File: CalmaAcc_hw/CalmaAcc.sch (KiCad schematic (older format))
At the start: 27 parts, among them Q1 MMBT2222

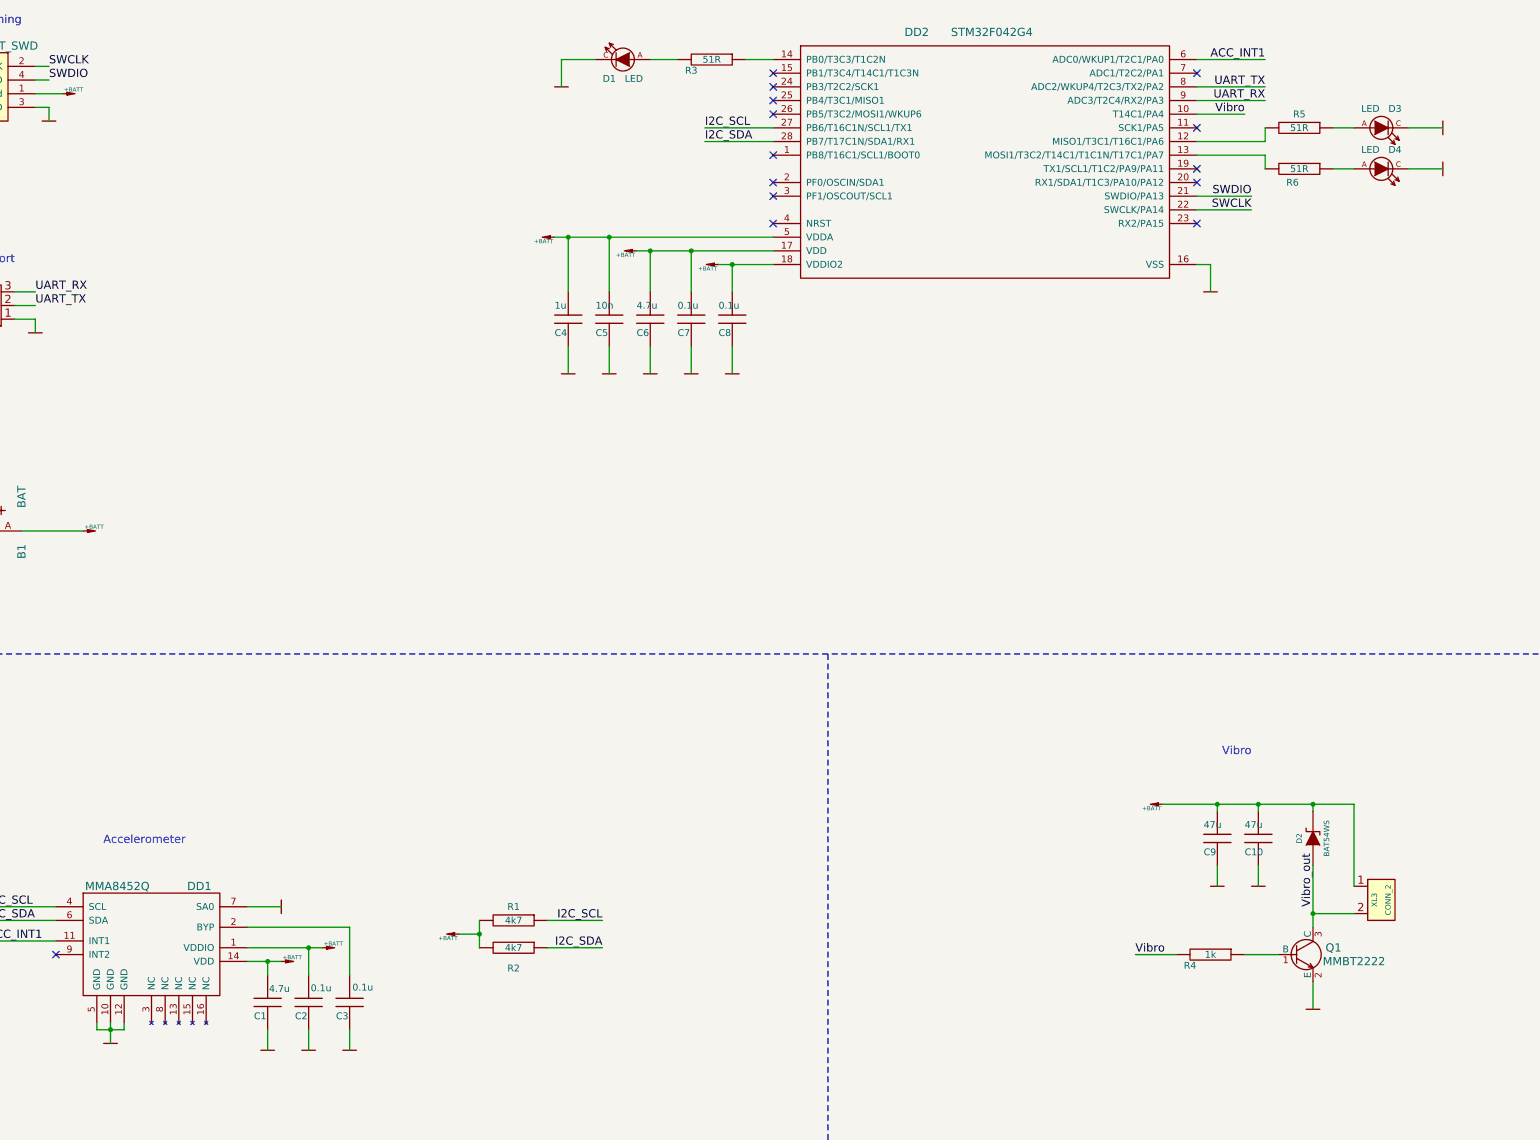
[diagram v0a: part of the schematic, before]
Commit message: +STM32F042F6
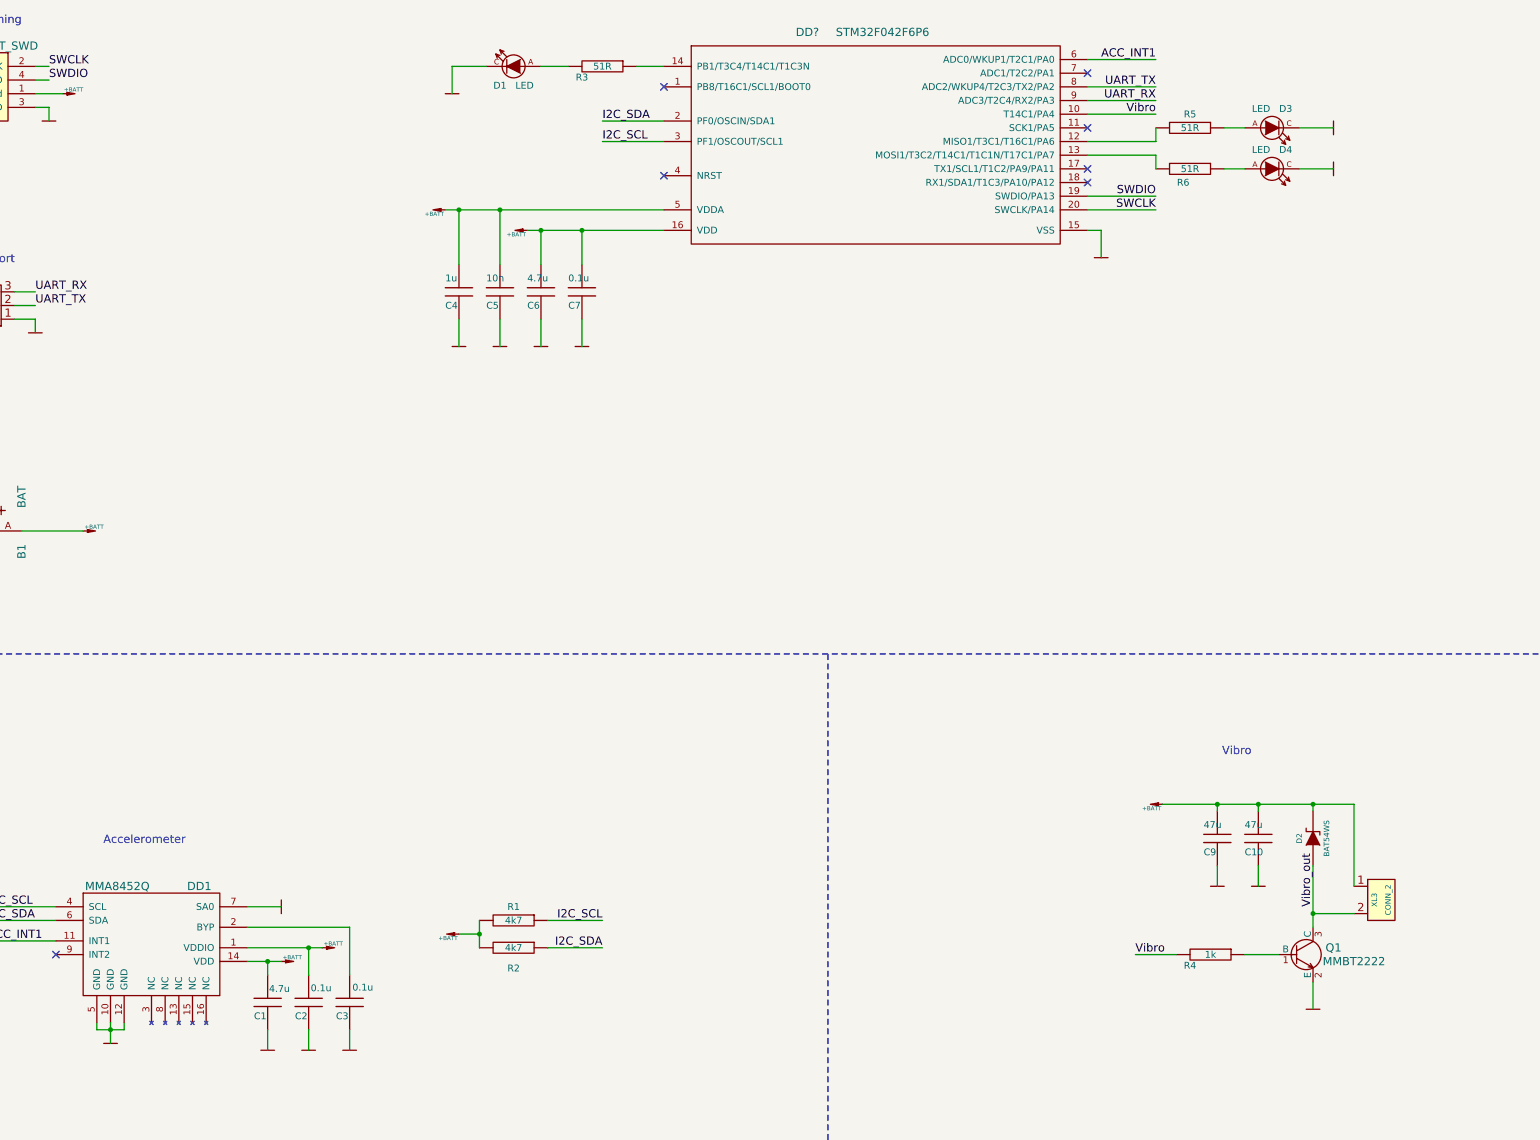
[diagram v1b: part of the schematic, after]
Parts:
- removed C8: 0.1u, Capacitors:CAP_0402, symbol C
- removed DD2: STM32F042G4, QFN_DFN:UFQFPN28, symbol STM32F042G4
- added DD?: STM32F042F6P6, symbol STM32F042F6P6
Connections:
- net +BATT: now also DD?.16 (VDD), DD?.5 (VDDA)
- net ACC_INT1: now also DD?.6 (ADC0/WKUP1/T2C1/PA0)
- net GND: now also DD?.15 (VSS)
- net I2C_SCL: now also DD?.3 (PF1/OSCOUT/SCL1)
- net I2C_SDA: now also DD?.2 (PF0/OSCIN/SDA1)
- net SWCLK: now also DD?.20 (SWCLK/PA14)
- net SWDIO: now also DD?.19 (SWDIO/PA13)
- net UART_RX: now also DD?.9 (ADC3/T2C4/RX2/PA3)
- net UART_TX: now also DD?.8 (ADC2/WKUP4/T2C3/TX2/PA2)
- net Vibro: now also DD?.10 (T14C1/PA4)
- net at R5.2: now also DD?.12 (MISO1/T3C1/T16C1/PA6)
- net at R6.2: now also DD?.13 (MOSI1/T3C2/T14C1/T1C1N/T17C1/PA7)
- net at R3.1: now also DD?.14 (PB1/T3C4/T14C1/T1C3N)
- no-connect marks 15 -> 8
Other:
- moved on the sheet: C4, C5, C6, C7, D1, D3, D4, R3, R5, R6
